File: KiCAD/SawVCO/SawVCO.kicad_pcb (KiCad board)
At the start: 2 copper layers, 94 x 73.7 mm, 46 parts, among them J1 PWR_IN, J10 Saw_Out, J2 Liner_FM, J3 PWR_OUT, J4 I_Ref, J5 I_Sink, J6 TP_GND, J7 Sync_In, J8 Saw_Out, J9 Saw_Out, Q1 2SA1015, U1 TL072, U2 TL072

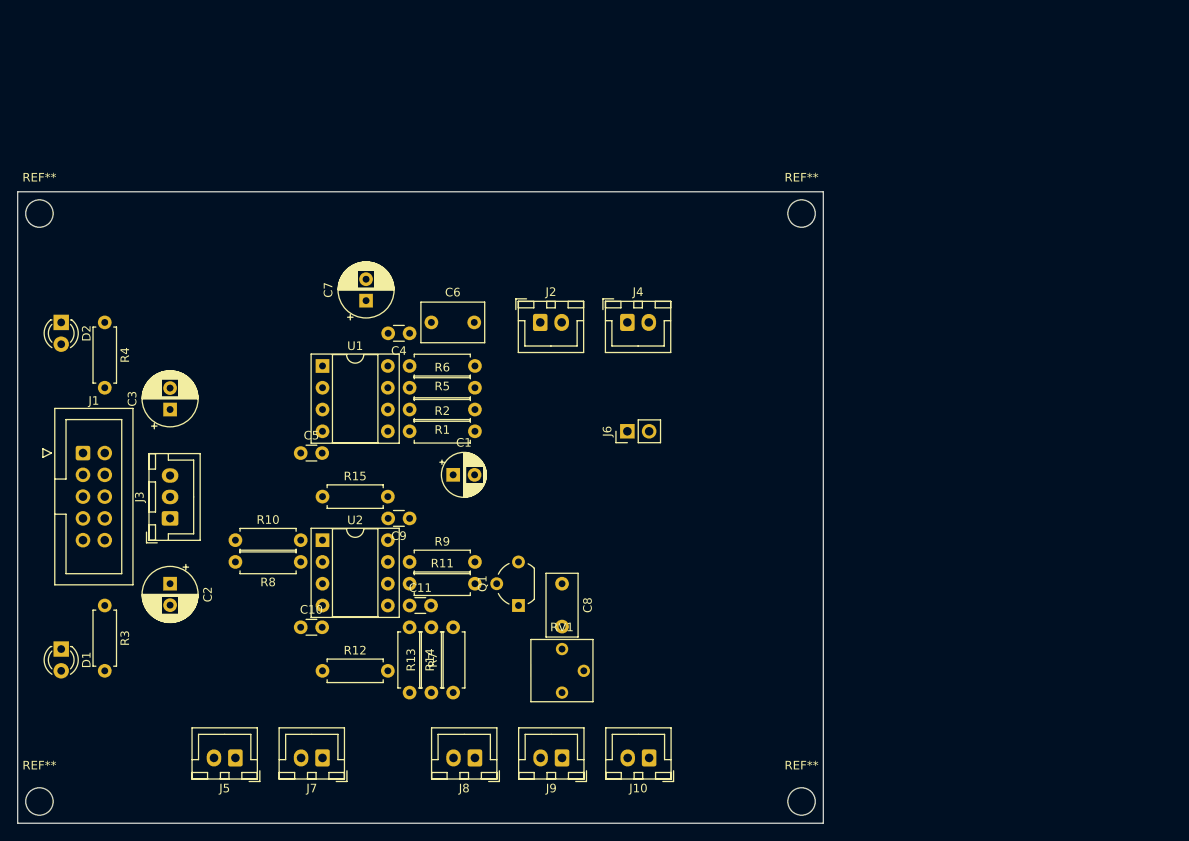
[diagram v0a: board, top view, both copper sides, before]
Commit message: Update
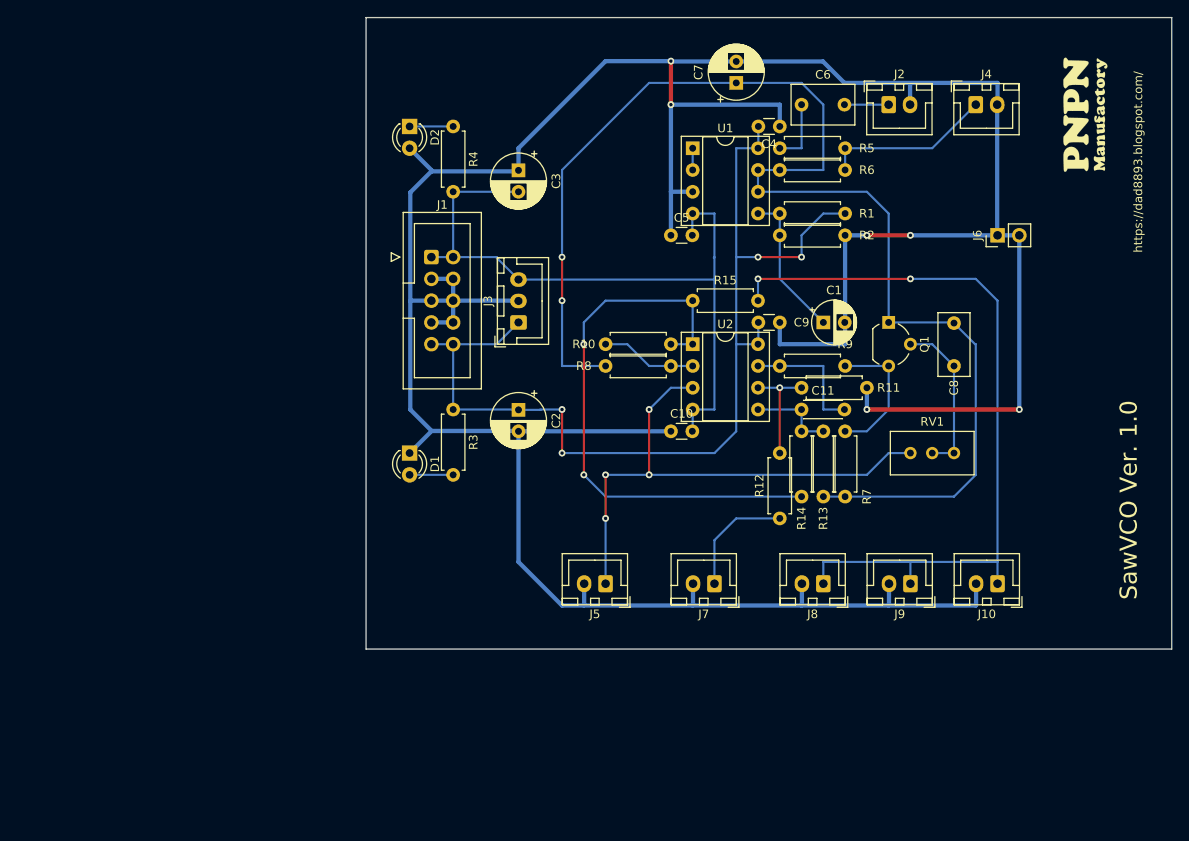
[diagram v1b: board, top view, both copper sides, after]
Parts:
- removed REF** (x4): MountingHole_3.2mm_M3, MountingHole:MountingHole_3.2mm_M3
- added G***: LOGO, myfootprint:Silk_PNPN_Manufactory_600dpi, F.Cu at (182.7, 72.3)
- C11: footprint Capacitor_THT:C_Disc_D3.0mm_W1.6mm_P2.50mm -> Capacitor_THT:C_Disc_D4.3mm_W1.9mm_P5.00mm
- RV1: value 5k -> 10k; footprint myfootprint:Potentiometer_Bourns_3362P_Vertical -> Potentiometer_THT:Potentiometer_Bourns_3296W_Vertical
- moved R12 56.2 mm to (147.3, 119.4), turned to 90 degrees
- moved Q1 54.4 mm to (160.0, 96.5), turned to 270 degrees
- moved RV1 53.6 mm to (167.6, 111.8)
- moved C8 52.3 mm to (167.6, 101.6), turned to 90 degrees
- moved R14 51.1 mm to (149.9, 109.2)
- moved C11 51.1 mm to (149.9, 106.7)
- moved R11 51.1 mm to (149.9, 104.1)
- moved R13 51.1 mm to (152.4, 116.8)
- moved R7 51.1 mm to (154.9, 116.8)
- moved C5 50.1 mm to (134.6, 86.4)
- moved C7 50.1 mm to (142.2, 68.6)
- moved C6 50.1 mm to (149.9, 71.1)
- moved R6 50.1 mm to (147.3, 78.7)
- moved R5 50.1 mm to (154.9, 76.2)
- moved U1 50.1 mm to (137.2, 76.2)
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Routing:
- net GND: track 0.00 -> 390.3 mm, vias 0 -> 6
- net /+5V: track 0.00 -> 155.7 mm, vias 0 -> 2
- net +12V: track 0.00 -> 117.5 mm, vias 0 -> 4
- net Net-(J10-Pad1): track 0.00 -> 90.0 mm, vias 0 -> 2
- net -12V: track 0.00 -> 82.9 mm
- net Net-(R10-Pad2): track 0.00 -> 65.6 mm, vias 0 -> 2
- net Net-(J5-Pad1): track 0.00 -> 63.1 mm, vias 0 -> 4
- net Net-(J4-Pad1): track 0.00 -> 19.9 mm
- net Net-(C8-Pad1): track 0.00 -> 18.8 mm
- net Net-(C1-Pad1): track 0.00 -> 17.3 mm
- net Net-(Q1-Pad3): track 0.00 -> 16.3 mm
- net Net-(C11-Pad2): track 0.00 -> 15.2 mm
- net Net-(J7-Pad1): track 0.00 -> 13.8 mm
- net Net-(R11-Pad1): track 0.00 -> 12.7 mm, vias 0 -> 1
- net Net-(R10-Pad1): track 0.00 -> 11.2 mm
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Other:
- board text added: "SawVCO Ver. 1.0"
- board text added: "https://dad8893.blogspot.com/"
